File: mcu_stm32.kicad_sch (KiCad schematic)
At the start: 49 parts, among them J11 Conn_01x03, J2 Conn_ARM_JTAG_SWD_20, J3 Conn_01x03, U4 STM32F407VETx, U5 24LC256, Y1 8 MHz, Y2 32k

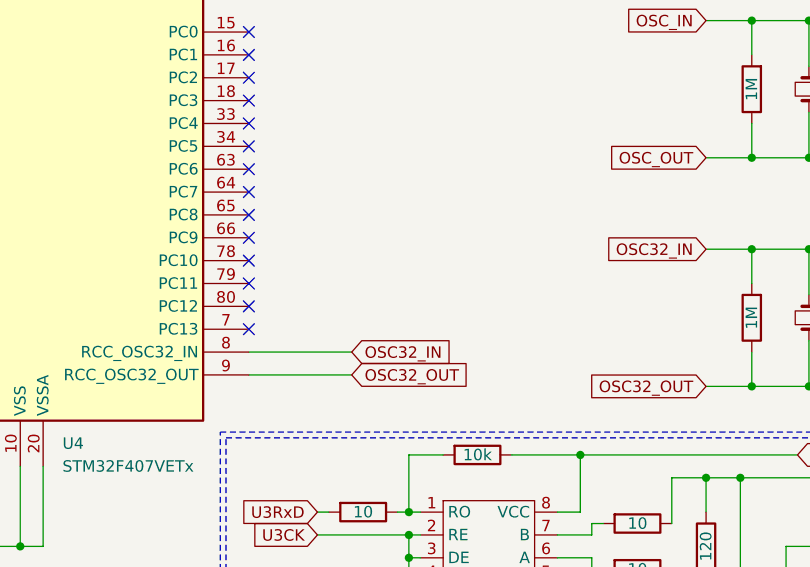
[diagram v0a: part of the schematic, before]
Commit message: redaction_11
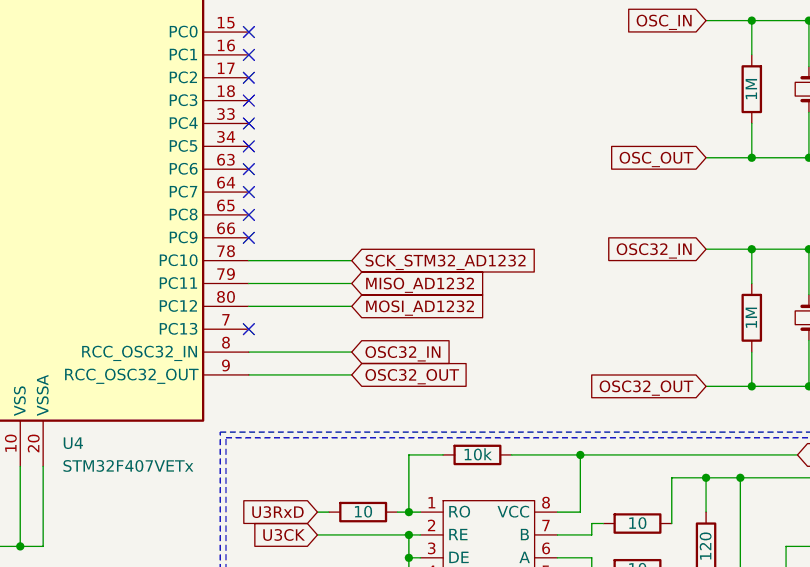
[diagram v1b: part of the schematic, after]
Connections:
- net SCK_STM32_AD1232: now reaches U4.78 (PC10)
- net MISO_AD1232: now reaches U4.79 (PC11)
- net MOSI_AD1232: now reaches U4.80 (PC12)
- no-connect marks 61 -> 58
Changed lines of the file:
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@@
 	)
 	(no_connect
-		(at 100.33 148.59)
-	)
-	(no_connect
 		(at 49.53 105.41)
 	)
@@
 	)
 	(no_connect
-		(at 100.33 151.13)
-	)
-	(no_connect
 		(at 100.33 46.99)
 	)
@@
 	)
 	(no_connect
-		(at 100.33 146.05)
-	)
-	(no_connect
 		(at 100.33 54.61)
 	)
@@
 	(wire
 		(pts
+			(xy 100.33 151.13) (xy 111.76 151.13)
+		)
+		(stroke
+			(width 0)
+			(type default)
+		)
+	)
+	(wire
+		(pts
 			(xy 222.25 83.82) (xy 222.25 121.92)
 		)
@@
 	(wire
 		(pts
+			(xy 100.33 148.59) (xy 111.76 148.59)
+		)
+		(stroke
+			(width 0)
+			(type default)
+		)
+	)
+	(wire
+		(pts
 			(xy 162.56 100.33) (xy 162.56 95.25)
 		)
@@
 	(wire
 		(pts
+			(xy 100.33 146.05) (xy 111.76 146.05)
+		)
+		(stroke
+			(width 0)
+			(type default)
+		)
+	)
+	(wire
+		(pts
 			(xy 162.56 144.78) (xy 162.56 149.86)
 		)
@@
 		)
 	)
+	(global_label "SCK_STM32_AD1232"
+		(shape input)
+		(at 111.76 146.05 0)
+		(fields_autoplaced yes)
+		(effects
+			(font
+				(size 1.27 1.27)
+			)
+			(justify left)
+		)
+		(property "Intersheetrefs" "${INTERSHEET_REFS}"
+			(at 133.674 146.05 0)
+			(hide yes)
+			(show_name no)
+			(do_not_autoplace no)
+			(effects
+				(font
+					(size 1.27 1.27)
+				)
+				(justify left)
+			)
+		)
+	)
 	(global_label "+3.3 VDD"
 		(shape input)
@@
 		)
 	)
+	(global_label "MOSI_AD1232"
+		(shape input)
+		(at 111.76 151.13 0)
+		(fields_autoplaced yes)
+		(effects
+			(font
+				(size 1.27 1.27)
+			)
+			(justify left)
+		)
+		(property "Intersheetrefs" "${INTERSHEET_REFS}"
+			(at 127.5056 151.13 0)
+			(hide yes)
+			(show_name no)
+			(do_not_autoplace no)
+			(effects
+				(font
+					(size 1.27 1.27)
+				)
+				(justify left)
+			)
+		)
+	)
 	(global_label "GND_0"
 		(shape input)
@@
 			(hide yes)
 			(show_name no)
+			(do_not_autoplace no)
+			(effects
+				(font
+					(size 1.27 1.27)
+				)
+				(justify left)
+			)
+		)
+	)
+	(global_label "MISO_AD1232"
+		(shape input)
+		(at 111.76 148.59 0)
+		(fields_autoplaced yes)
+		(effects
+			(font
+				(size 1.27 1.27)
+			)
+			(justify left)
+		)
+		(property "Intersheetrefs" "${INTERSHEET_REFS}"
+			(at 127.5056 148.59 0)
+			(hide yes)
+			(show_name no)
